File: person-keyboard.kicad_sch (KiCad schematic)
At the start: 36 parts, among them J1 USB_C_Receptacle_USB2.0_16P, SW106 SW_Push, SW107 SW_Push, U1 RP2040, U2 AMS1117-3.3, U3 W25Q128JVS, U4 PRTR5V0U2X, Y1 ABM8-272-T3

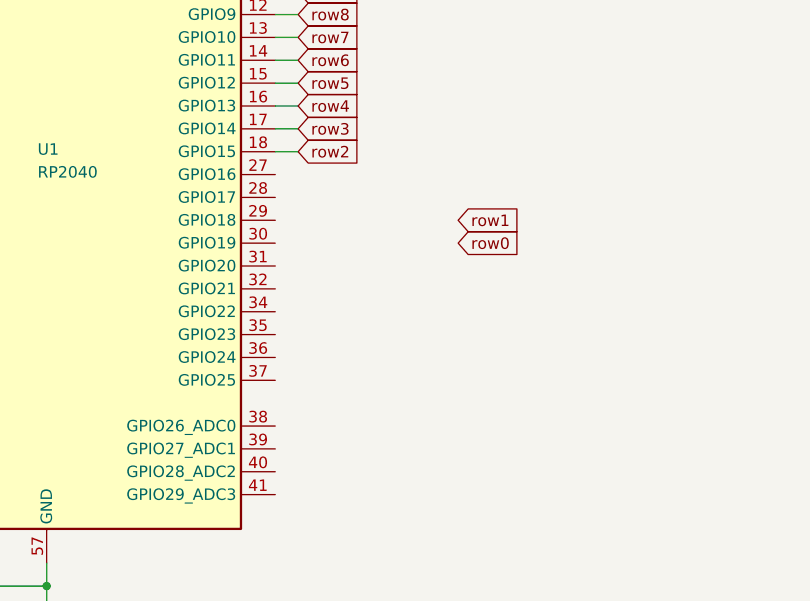
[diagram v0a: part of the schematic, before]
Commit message: Started Main matrix
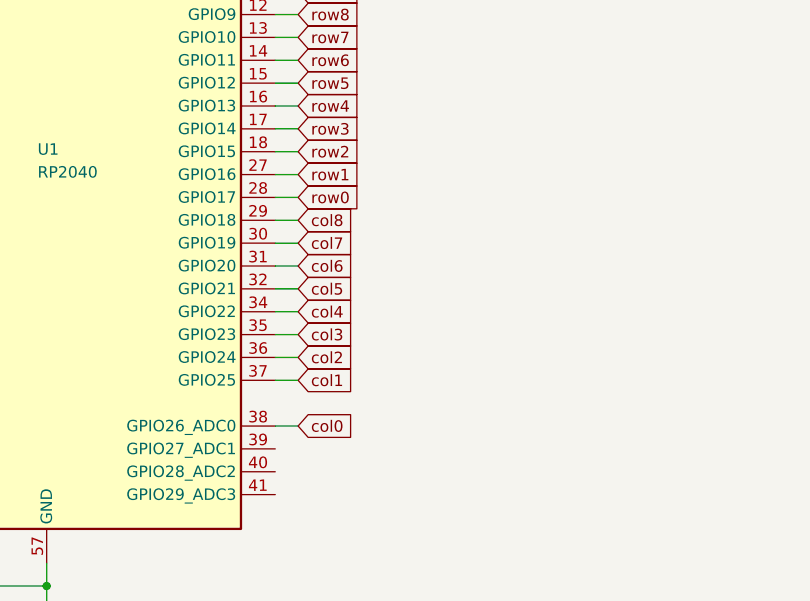
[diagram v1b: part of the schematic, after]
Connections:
- net row0: now also U1.28 (GPIO17)
- net row1: now also U1.27 (GPIO16)
- net col8: now reaches U1.29 (GPIO18)
- net col7: now reaches U1.30 (GPIO19)
- net col6: now reaches U1.31 (GPIO20)
- net col5: now reaches U1.32 (GPIO21)
- net col4: now reaches U1.34 (GPIO22)
- net col3: now reaches U1.35 (GPIO23)
- net col2: now reaches U1.36 (GPIO24)
- net col1: now reaches U1.37 (GPIO25)
- net col0: now reaches U1.38 (GPIO26_ADC0)
